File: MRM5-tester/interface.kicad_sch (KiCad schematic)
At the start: 27 parts, among them J1 Conn_01x05, J2 Conn_01x02, J3 Conn_01x05, J4 GSB1C41110SSHR, J5 Conn_01x02, J6 Conn_01x02, Q5 MMBT3906-TP, Q6 MMBT3906-TP, U1 CP2102N-A02-GQFN20

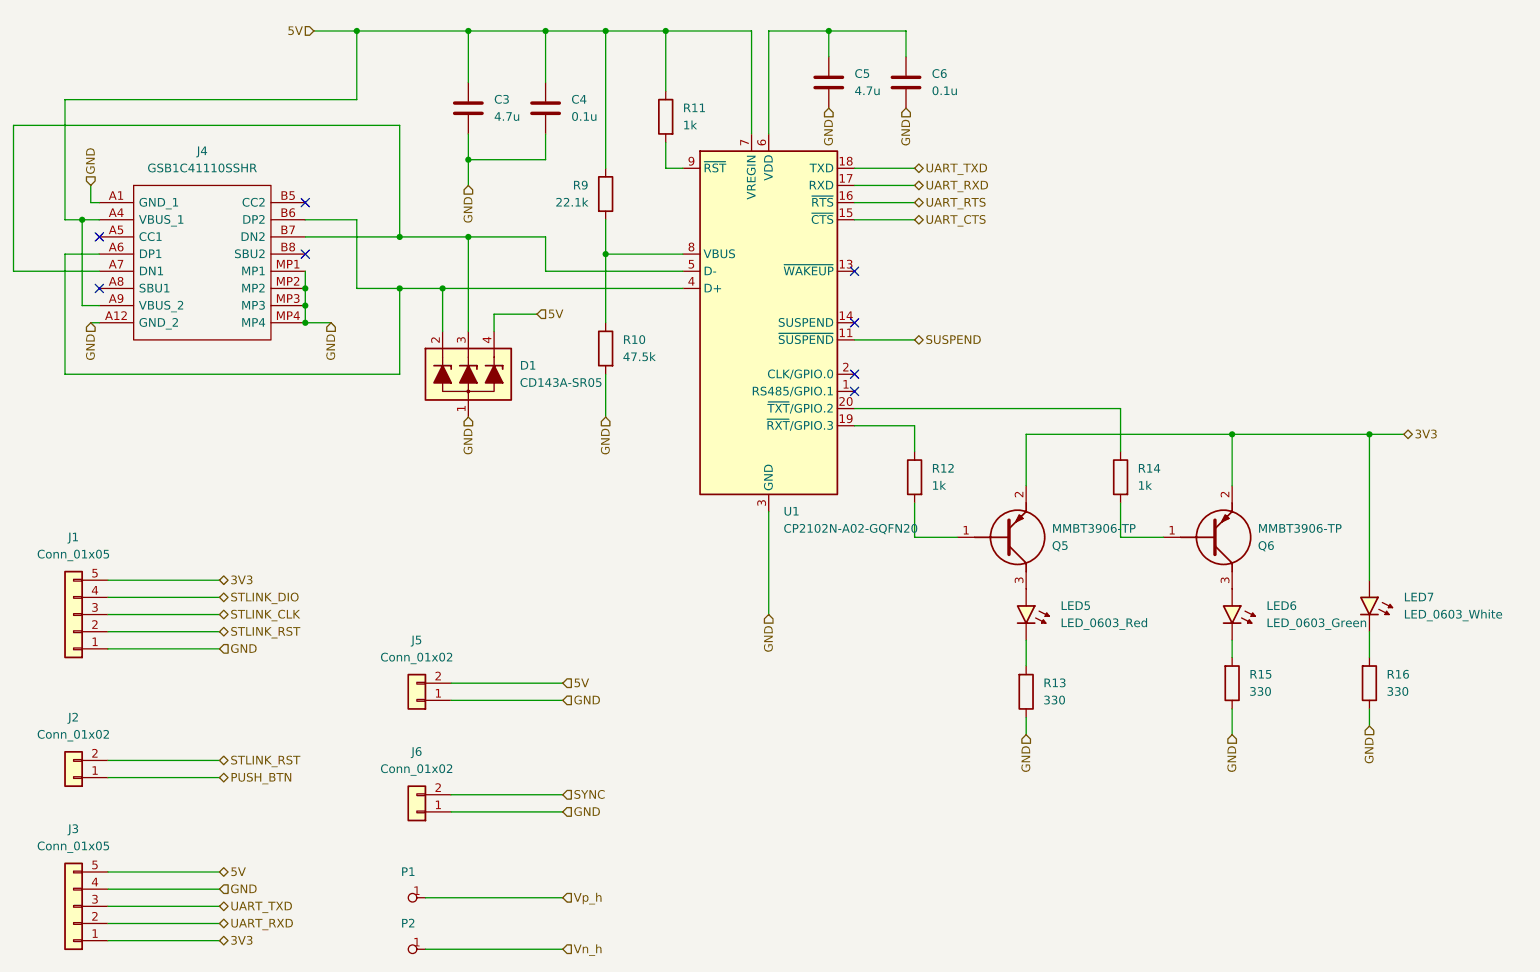
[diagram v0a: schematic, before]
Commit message: case updated
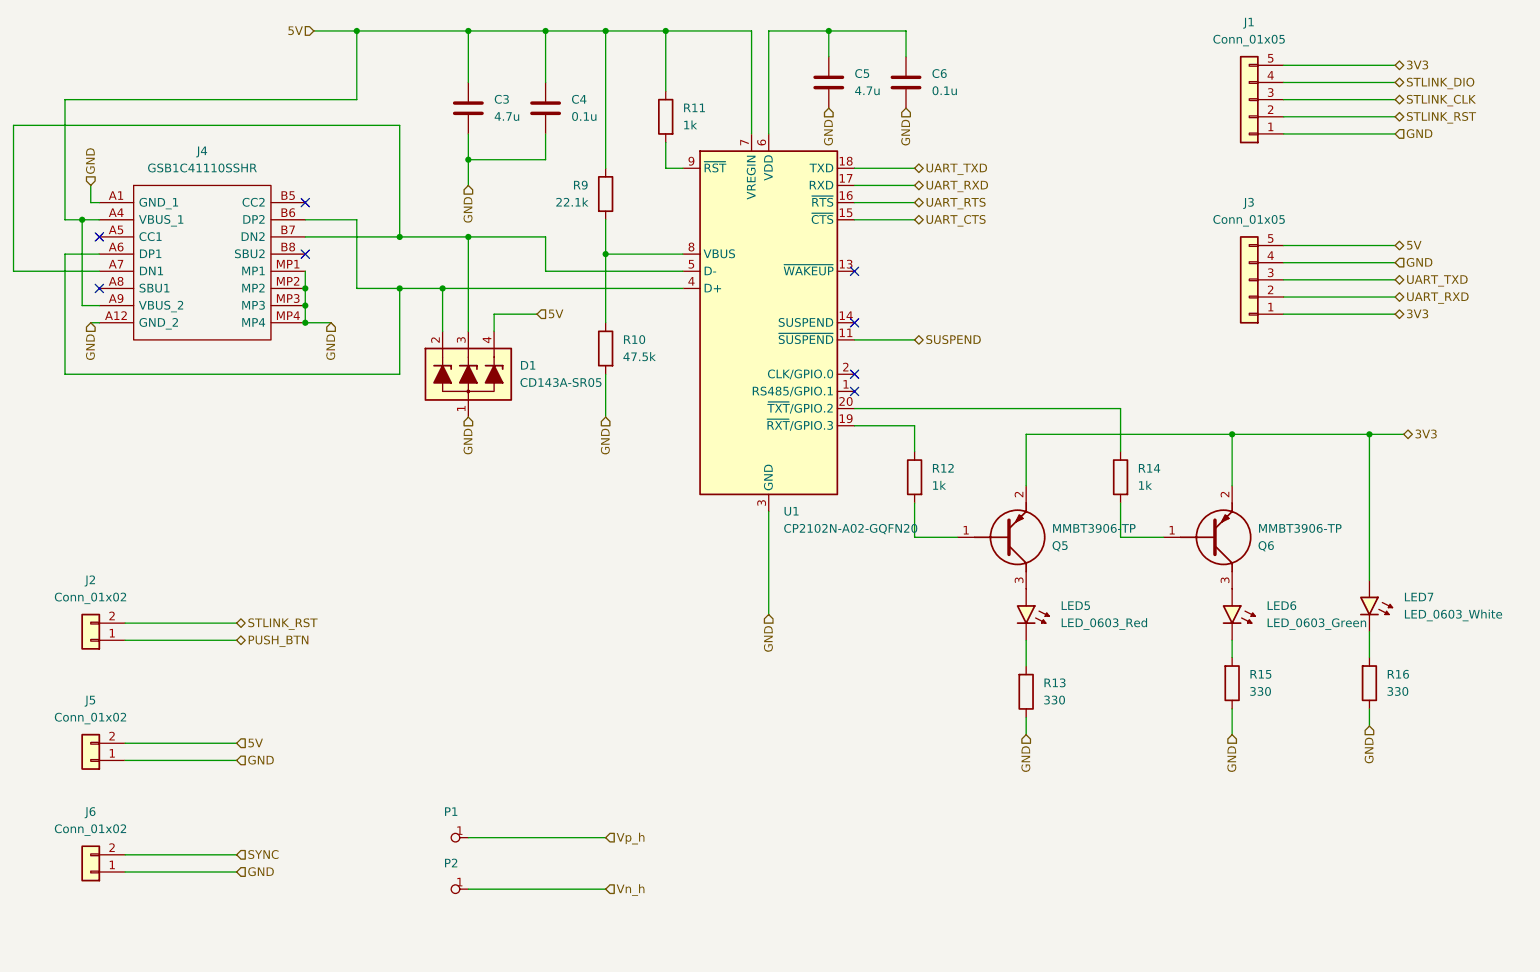
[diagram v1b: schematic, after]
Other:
- moved on the sheet: J1, J2, J3, J5, J6, P1, P2
